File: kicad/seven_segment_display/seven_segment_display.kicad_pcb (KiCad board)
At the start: 2 copper layers, 85.7 x 54 mm, 11 parts, among them J3 Conn_01x12_Pin, U1 74AHC595

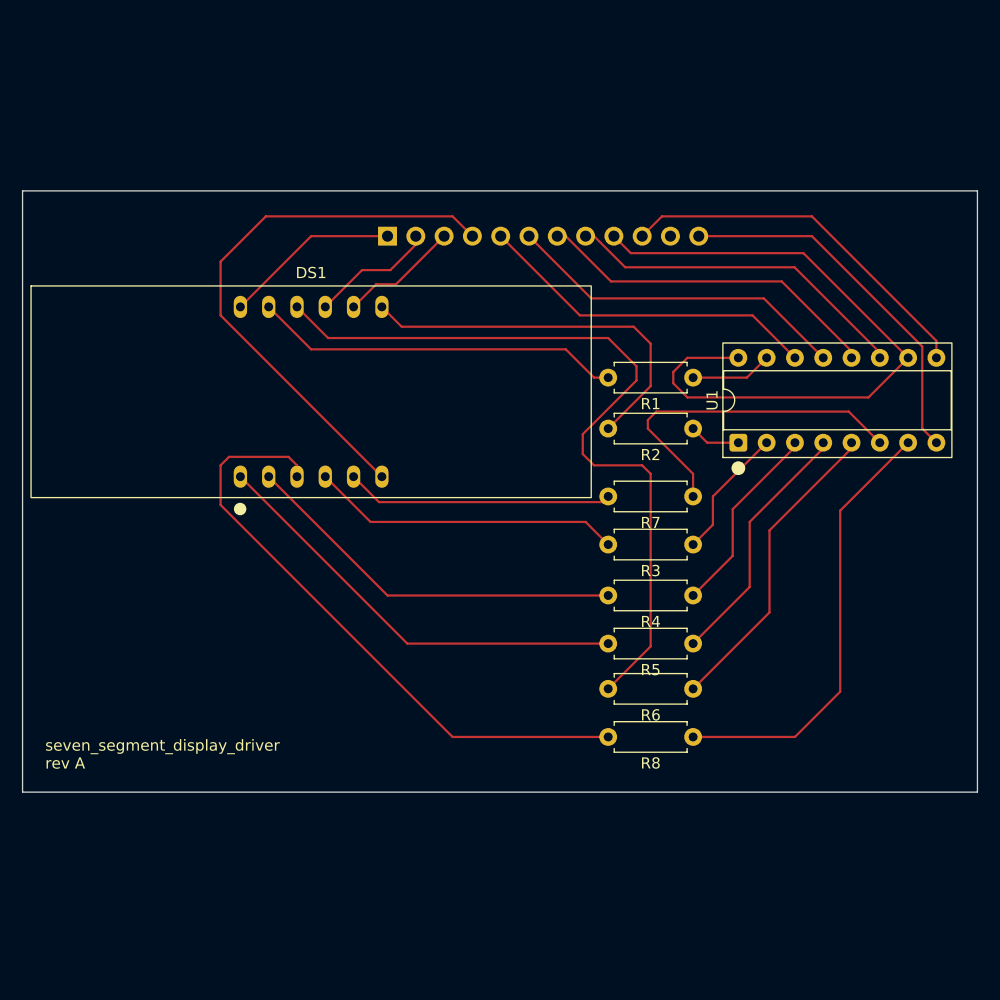
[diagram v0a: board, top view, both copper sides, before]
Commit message: final pcb design completed
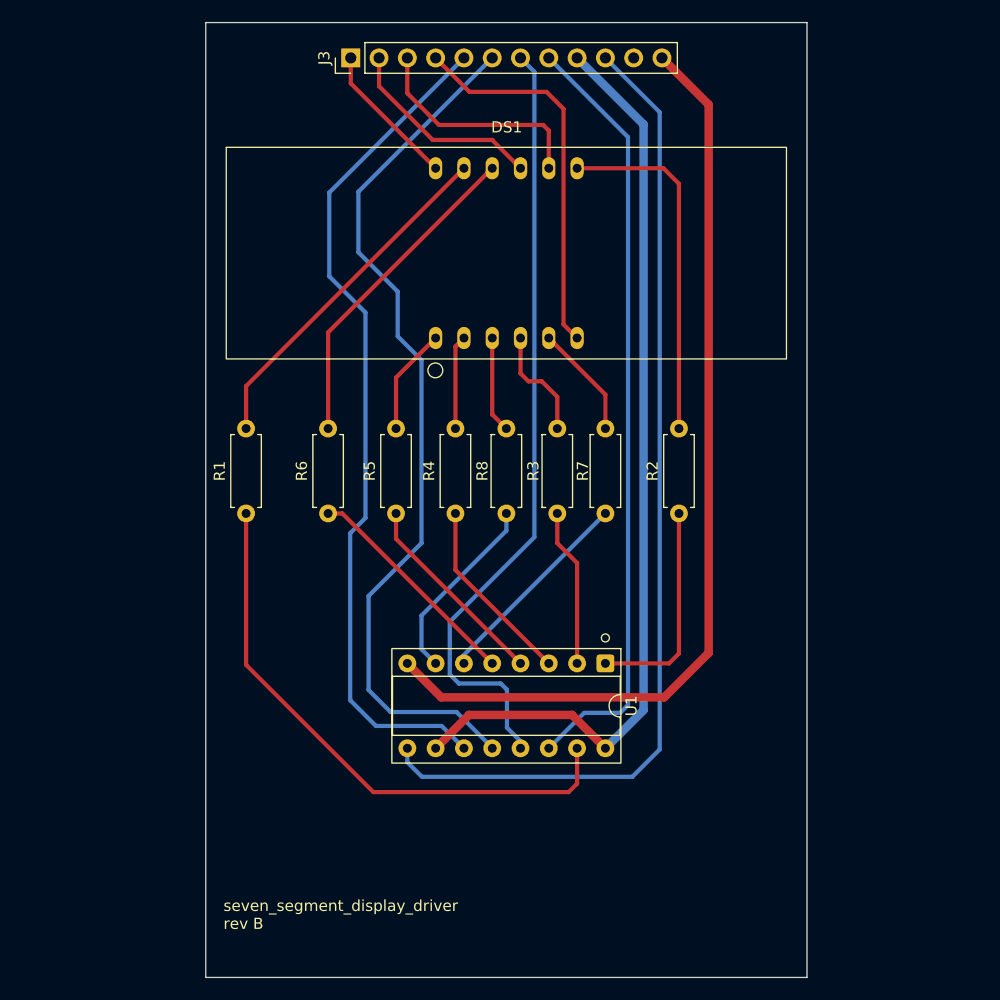
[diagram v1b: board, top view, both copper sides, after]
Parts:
- J3: moved to F.Cu
- moved R1 41.9 mm to (122.7, 99.3), turned to 90 degrees
- moved R6 36.4 mm to (130.0, 99.3), turned to 90 degrees
- moved R5 29.1 mm to (136.1, 99.3), turned to 90 degrees
- moved R8 26.1 mm to (146.1, 99.3), turned to 90 degrees
- moved U1 23.1 mm to (154.9, 112.8), turned to -90 degrees
- moved R4 22.6 mm to (141.5, 99.3), turned to 90 degrees
- moved DS1 21.5 mm to (146.1, 75.9)
- moved J3 16.3 mm to (132.1, 58.4), turned to 90 degrees
- moved R3 12.5 mm to (150.6, 99.3), turned to 90 degrees
- moved R7 8.02 mm to (154.9, 99.3), turned to 90 degrees
- moved R2 7.73 mm to (161.5, 99.3), turned to 90 degrees
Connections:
- J3 pad 5: /SER -> /CLK
- J3 pad 6: /~OE -> /LATCH
- J3 pad 7: /LATCH -> /~OE
- J3 pad 8: /CLK -> /SER
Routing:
- net /QH': track 33.3 -> 89.6 mm
- net GND: track 33.3 -> 85.1 mm
- net /LATCH: track 31.3 -> 79.3 mm
- net Net-(DS1-D.P.): track 55.5 -> 8.65 mm
- net /CLK: track 31.2 -> 76.6 mm
- net Net-(U1-QA): track 7.34 -> 51.5 mm
- net Net-(DS1-F): track 70.3 -> 29.5 mm
- net /~OE: track 30.9 -> 70.5 mm
- net /SER: track 30.9 -> 69.8 mm
- net Net-(DS1-E): track 39.2 -> 9.60 mm
- net Net-(DS1-D): track 34.9 -> 8.44 mm
- net Net-(U1-QH): track 39.8 -> 17.1 mm
- net +5V: track 61.4 -> 83.6 mm
- net Net-(DS1-C): track 27.9 -> 10.2 mm
- net /DIG4: track 50.6 -> 34.5 mm
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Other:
- board size 85.7 x 54 mm -> 54 x 85.7 mm
- board text added: "seven_segment_display_driver rev B"
- board text removed: "seven_segment_display_driver rev A"
